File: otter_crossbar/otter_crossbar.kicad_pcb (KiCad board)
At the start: 4 copper layers, 166 x 19 mm, 13 parts, among them J1 Conn_02x12_Counter_Clockwise, J2 Conn_02x12_Counter_Clockwise, J3 Conn_02x12_Counter_Clockwise, J4 Conn_02x08_Odd_Even, J5 Conn_02x08_Odd_Even

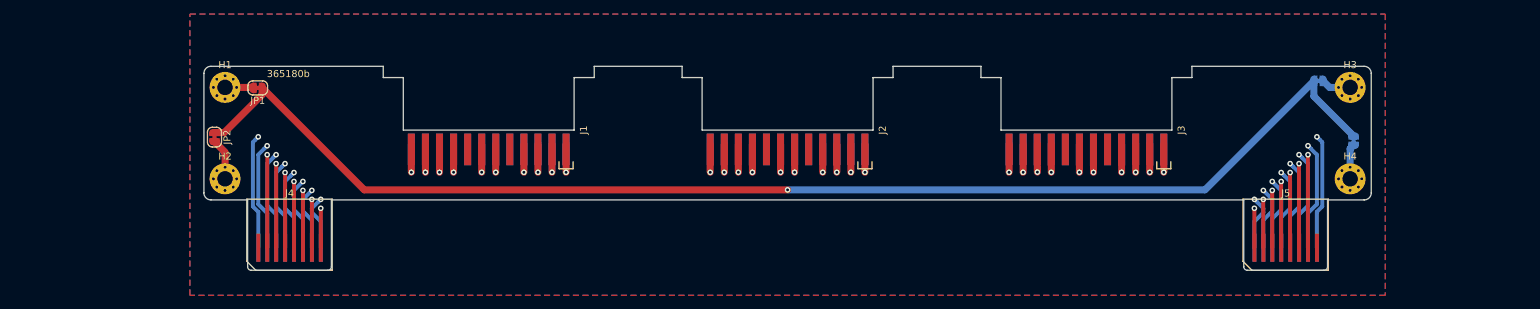
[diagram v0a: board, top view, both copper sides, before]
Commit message: wip on crossbars
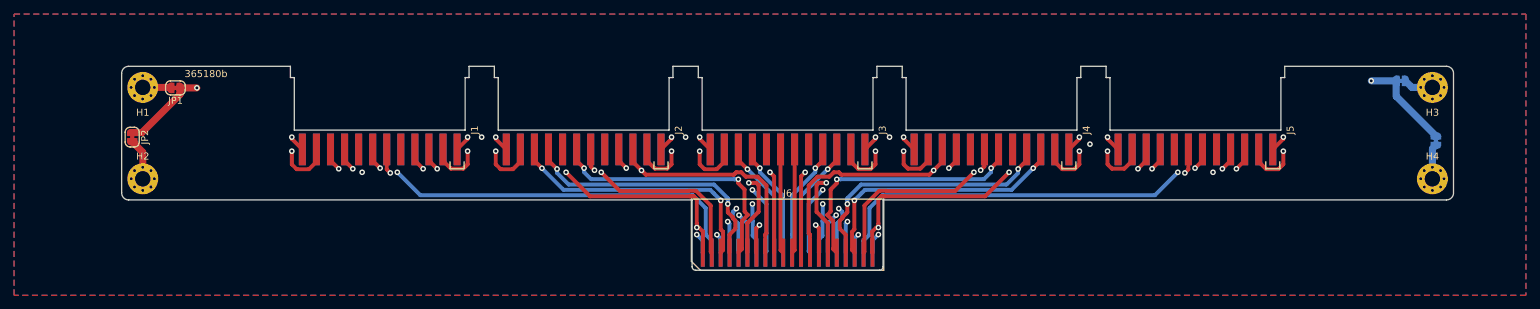
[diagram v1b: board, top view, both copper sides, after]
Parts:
- added J6: Conn_02x20_Odd_Even, custom:Samtec_MECF-20-0_-NP-L-DV_2x20_P1.27mm_Edge_mod, F.Cu at (0.00, -5.00)
- J4, J5: value Conn_02x08_Odd_Even -> Conn_02x12_Counter_Clockwise; footprint custom:Samtec_MECF-08-0_-NP-L-DV_2x08_P1.27mm_Edge_mod -> custom:PinSocket_2x12_P2.00mm_Vertical_EDGE
- moved J4 100.9 mm to (29.0, -19.9)
- moved J3 42.5 mm to (0.00, -19.9)
- moved J2 29.0 mm to (-29.0, -19.9)
- moved J5 19.7 mm to (58.0, -19.9)
- moved J1 15.5 mm to (-58.0, -19.9)
- moved H1 11.7 mm to (-91.7, -26.0)
- moved H2 11.7 mm to (-91.7, -13.0)
- moved H3 11.7 mm to (91.7, -26.0)
- moved H4 11.7 mm to (91.7, -13.0)
- moved JP1 11.7 mm to (-87.0, -25.9)
- moved JP2 11.7 mm to (-93.2, -18.9)
- moved JP3 11.7 mm to (87.2, -26.9)
- moved JP4 11.7 mm to (92.2, -18.4)
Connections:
- J1 pad 1: /C1 -> /E1
- J1 pad 11: /C6 -> /E6
- J1 pad 13: /C7 -> /E7
- J1 pad 17: /C9 -> /E9
- J1 pad 19: /C10 -> /E10
- J1 pad 21: /C11 -> /E2
- J1 pad 23: /C12 -> /E1
- J1 pad 3: /C2 -> /E2
- J1 pad 5: /C3 -> /E3
- J1 pad 7: /C4 -> /E4
- J2 pad 1: /B1 -> /D1
- J2 pad 11: /B6 -> /D6
- J2 pad 13: /B7 -> /D7
- J2 pad 17: /B9 -> /D9
- J2 pad 19: /B10 -> /D10
- J2 pad 21: /B11 -> /D2
- J2 pad 23: /B12 -> /D1
- J2 pad 3: /B2 -> /D2
- J2 pad 5: /B3 -> /D3
- J2 pad 7: /B4 -> /D4
- J3 pad 1: /A1 -> /C1
- J3 pad 11: /A6 -> /C6
- J3 pad 13: /A7 -> /C7
- J3 pad 17: /A9 -> /C9
- J3 pad 19: /A10 -> /C10
- J3 pad 21: /A11 -> /C2
- J3 pad 23: /A12 -> /C1
- J3 pad 3: /A2 -> /C2
- J3 pad 5: /A3 -> /C3
- J3 pad 7: /A4 -> /C4
- J4 pad 1: GND -> /B1
- J4 pad 10: /C7 -> (no net)
- J4 pad 11: /B12 -> /B6
- J4 pad 12: /C6 -> (no net)
- J4 pad 13: /C1 -> /B7
- J4 pad 14: /C4 -> (no net)
- J4 pad 15: /C2 -> (no net)
- J4 pad 16: /C3 -> (no net)
- J4 pad 2: /C12 -> (no net)
- J4 pad 3: /B7 -> /B2
- J4 pad 4: /C11 -> (no net)
- J4 pad 5: /B9 -> /B3
- J4 pad 6: /C10 -> (no net)
- J4 pad 7: /B10 -> /B4
- J4 pad 8: /C9 -> (no net)
- J4 pad 9: /B11 -> (no net)
- J5 pad 1: /A11 -> /A1
- J5 pad 10: /A4 -> (no net)
- J5 pad 11: /B4 -> /A6
- J5 pad 12: /A3 -> (no net)
- J5 pad 13: /B6 -> /A7
- J5 pad 14: /A2 -> (no net)
- J5 pad 15: GND -> (no net)
- J5 pad 16: /A1 -> (no net)
- J5 pad 2: /A10 -> (no net)
- J5 pad 3: /A12 -> /A2
- J5 pad 4: /A9 -> (no net)
- J5 pad 5: /B1 -> /A3
- J5 pad 6: /A7 -> (no net)
- J5 pad 7: /B2 -> /A4
- J5 pad 8: /A6 -> (no net)
- J5 pad 9: /B3 -> (no net)
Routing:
- net /E2: track 0.00 -> 96.2 mm, vias 0 -> 3
- net /E1: track 0.00 -> 93.0 mm, vias 0 -> 4
- net /B11: track 77.2 -> 0.00 mm, vias 2 -> 0
- net /B12: track 72.6 -> 0.00 mm, vias 2 -> 0
- net /D2: track 0.00 -> 67.8 mm, vias 0 -> 3
- net GND: track 182.1 -> 114.5 mm, vias 1 -> 6
- net /E10: track 0.00 -> 65.0 mm, vias 0 -> 2
- net /E9: track 0.00 -> 64.5 mm, vias 0 -> 2
- net /E7: track 0.00 -> 63.6 mm, vias 0 -> 2
- net /E6: track 0.00 -> 63.4 mm, vias 0 -> 2
- net /D1: track 0.00 -> 63.1 mm, vias 0 -> 4
- net /E4: track 0.00 -> 59.3 mm, vias 0 -> 2
- net /E3: track 0.00 -> 59.1 mm, vias 0 -> 2
- net /C3: track 75.9 -> 16.8 mm, vias 2 -> 1
- net /B6: track 93.1 -> 37.6 mm
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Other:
- board size 166 x 19 mm -> 189.4 x 19 mm
